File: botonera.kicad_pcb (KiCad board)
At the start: 2 copper layers, 139 x 73 mm, 17 parts, among them J1 VCC, J2 RST, J3 BUTTON1, J4 BUTTON2, J5 LIGHT1, J6 LIGHT2, K1 SUNHOLD_RAS_Form_C, K2 SUNHOLD_RAS_Form_C, K3 SUNHOLD_RAS_Form_C, M1 MOUNTING-HOLE, M2 MOUNTING-HOLE, M3 MOUNTING-HOLE, M4 MOUNTING-HOLE

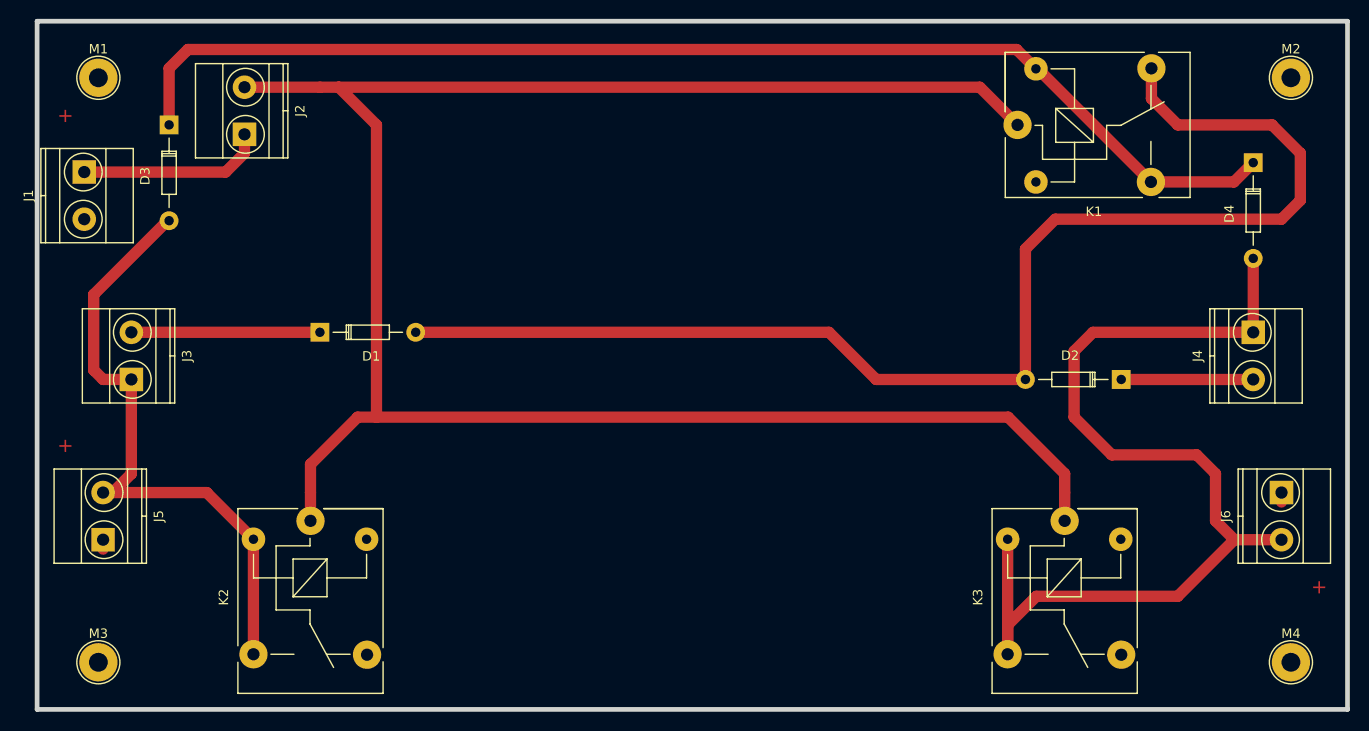
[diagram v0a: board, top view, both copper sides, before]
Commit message: esquematico y pcb generado
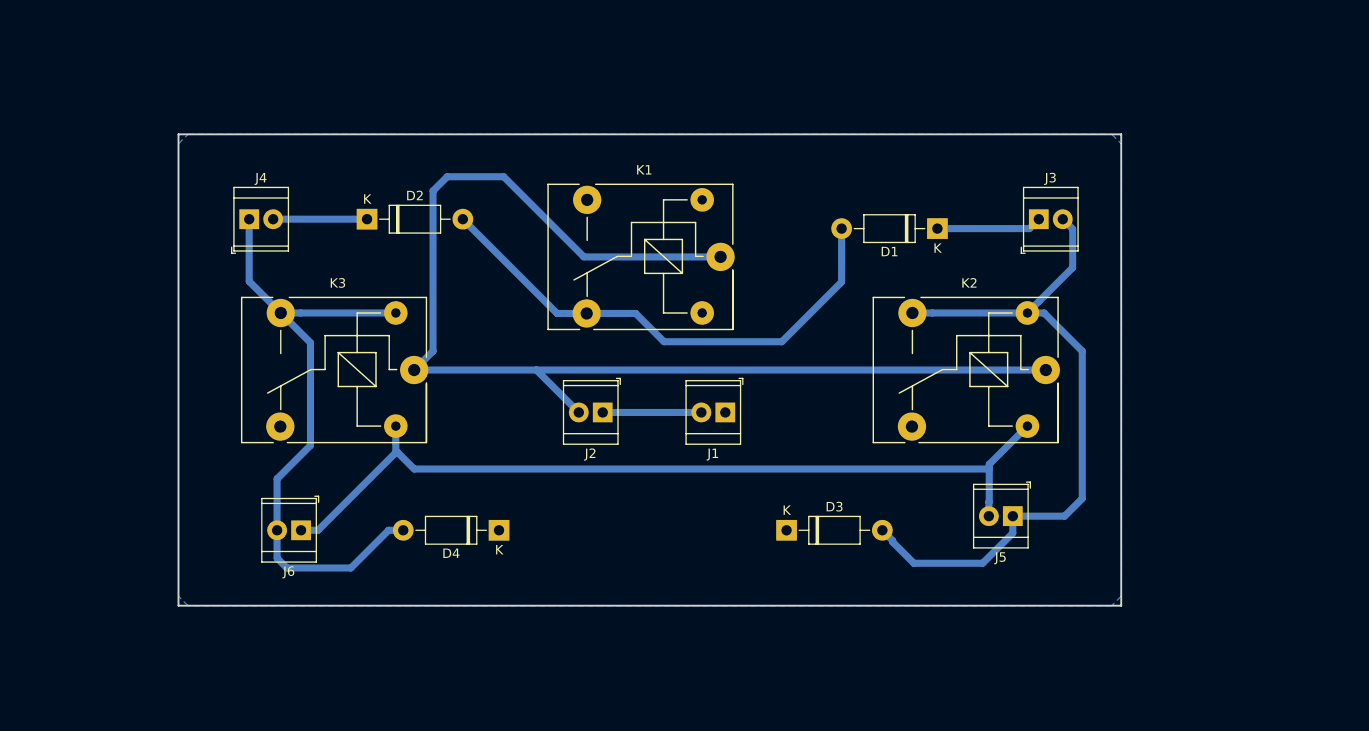
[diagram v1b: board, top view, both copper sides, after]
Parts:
- removed M1, M2, M3, M4: MOUNTING-HOLE, Connect:1pin
- D1, D2, D3, D4: footprint Diodes_ThroughHole:Diode_DO-35_SOD27_Horizontal_RM10 -> Diode_THT:D_DO-41_SOD81_P10.16mm_Horizontal
- J1, J2, J3, J4, J5, J6: footprint Terminal_Blocks:TerminalBlock_Pheonix_MKDS1.5-2pol -> TerminalBlock_TE-Connectivity:TerminalBlock_TE_282834-2_1x02_P2.54mm_Horizontal
- K1: value SUNHOLD_RAS_Form_C -> MAIN
- K2: value SUNHOLD_RAS_Form_C -> PLY1
- K3: value SUNHOLD_RAS_Form_C -> PLY2
- moved J4 107.2 mm to (72.5, 71.0), turned to 0 degrees
- moved J6 104.1 mm to (78.0, 104.0), turned to 180 degrees
- moved J3 97.7 mm to (156.3, 71.0), turned to 0 degrees
- moved J5 96.5 mm to (153.5, 102.5), turned to 180 degrees
- moved D4 89.0 mm to (99.0, 104.0), turned to 180 degrees
- moved D2 81.8 mm to (85.0, 71.0), turned to 0 degrees
- moved K2 79.6 mm to (157.0, 87.0), turned to 180 degrees
- moved D3 78.4 mm to (129.5, 104.0), turned to 0 degrees
- moved J1 72.6 mm to (123.0, 91.5), turned to 180 degrees
- moved K3 70.8 mm to (90.0, 87.0), turned to 180 degrees
- moved D1 66.4 mm to (145.5, 72.0), turned to 180 degrees
- moved J2 48.1 mm to (110.0, 91.5), turned to 180 degrees
- moved K1 34.5 mm to (122.5, 75.0), turned to 180 degrees
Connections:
- D3 pad 1: Net-(D3-Pad1) -> GND
- D4 pad 1: Net-(D3-Pad1) -> GND
- J1 pad 1: /Vcc1 -> GND
- J1 pad 2: GND -> +5V
- J2 pad 1: /Vcc1 -> +5V
- J3 pad 1: /BUTTON1_2 -> /BUTTON1_1
- J3 pad 2: /BUTTON1_1 -> /BUTTON1_2
- J5 pad 1: GND -> /BUTTON1_2
- J5 pad 2: /BUTTON1_2 -> Net-(J5-Pad2)
- J6 pad 1: GND -> Net-(J5-Pad2)
- K1 pad 2: Net-(D3-Pad1) -> GND
- K1 pad 5: Net-(D3-Pad1) -> GND
- K2 pad 2: GND -> Net-(J5-Pad2)
- K3 pad 2: GND -> Net-(J5-Pad2)
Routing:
- net Net-(D3-Pad1): track 128.6 -> 0.00 mm
- net Net-(J5-Pad2): track 0.00 -> 91.2 mm
- net /Vcc2: track 215.9 -> 127.8 mm
- net Net-(D1-Pad2): track 138.4 -> 53.9 mm
- net /BUTTON2_2: track 108.1 -> 67.8 mm
- net /Vcc1: track 19.8 -> 0.00 mm
- net +5V: track 0.00 -> 10.5 mm
- net /BUTTON1_1: track 20.0 -> 11.2 mm
- net /BUTTON1_2: track 68.7 -> 74.3 mm
- net /BUTTON2_1: track 14.0 -> 9.96 mm
- net GND: track 2.07 -> 0.00 mm
- added copper zone on B.Cu, net GND
- removed copper zone on F.Cu, net GND
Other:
- board size 139 x 73 mm -> 100 x 50 mm
- net class Default: trace_width 1.2 -> 0.75; via_dia 1.2 -> 0.8; via_drill 1 -> 0.4
- board text removed: "+"
- board text removed: "alto: 73 ancho: 139"
- board text removed: "orificios: largo: 127 mm alto: 62 mm"
